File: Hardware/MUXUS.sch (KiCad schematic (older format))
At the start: 120 parts, among them J1 USB_C_Receptacle_USB2.0, J2 USB_B, J3 USB_A, J4 USB_B, J5 USB_A, J6 STDC14, J7 USB_B, J8 USB_A, SW1 USER, SW2 RESET, U1 USBLC6-4SC6, U10 AP2151W, U11 AOZ1212AI, U12 USBLC6-2SC6, U13 USBLC6-2SC6, U14 AP2151W, U2 USB2504A-JT, U3 USBLC6-2SC6, U4 USBLC6-2SC6, U5 AP2151W, U6 TS3USBCA420RSVR, U7 STM32G431K8T6, U8 USBLC6-2SC6, U9 USBLC6-2SC6, Y1 ATS240C

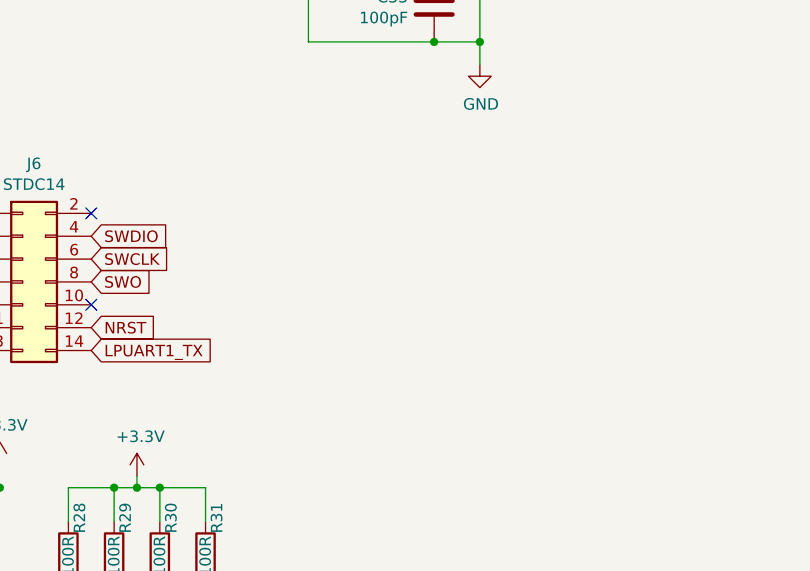
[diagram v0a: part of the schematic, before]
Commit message: DEBUG connectors and VIAS
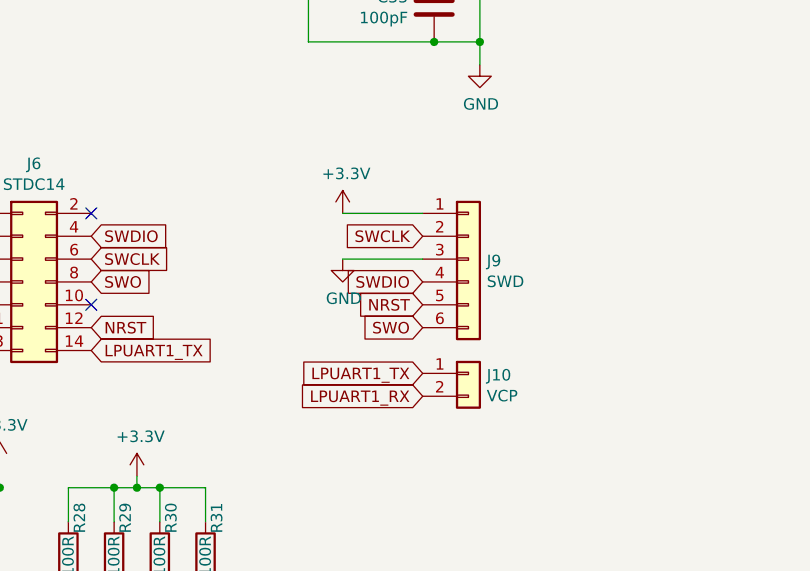
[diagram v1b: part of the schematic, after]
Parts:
- added J10: VCP, Connector_PinHeader_2.54mm:PinHeader_1x02_P2.54mm_Vertical, symbol Connector_Generic:Conn_01x02
- added J9: SWD, Connector_PinHeader_2.54mm:PinHeader_1x06_P2.54mm_Vertical, symbol Connector_Generic:Conn_01x06
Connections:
- net +3V3: now also J9.1 (Pin_1)
- net GND: now also J9.3 (Pin_3)
- net LPUART1_RX: now also J10.2 (Pin_2)
- net LPUART1_TX: now also J10.1 (Pin_1)
- net NRST: now also J9.5 (Pin_5)
- net SWCLK: now also J9.2 (Pin_2)
- net SWDIO: now also J9.4 (Pin_4)
- net SWO: now also J9.6 (Pin_6)
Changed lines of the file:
@@
 	2400 4350 2600 4350
 Connection ~ 2400 4650
+$Comp
+L Connector_Generic:Conn_01x06 J9
+U 1 1 615B40A3
+P 12450 8450
+F 0 "J9" H 12530 8442 50  0000 L CNN
+F 1 "SWD" H 12530 8351 50  0000 L CNN
+F 2 "Connector_PinHeader_2.54mm:PinHeader_1x06_P2.54mm_Vertical" H 12450 8450 50  0001 C CNN
+F 3 "~" H 12450 8450 50  0001 C CNN
+	1    12450 8450
+	1    0    0    -1
+$EndComp
+$Comp
+L Connector_Generic:Conn_01x02 J10
+U 1 1 615B75B8
+P 12450 8950
+F 0 "J10" H 12530 8942 50  0000 L CNN
+F 1 "VCP" H 12530 8851 50  0000 L CNN
+F 2 "Connector_PinHeader_2.54mm:PinHeader_1x02_P2.54mm_Vertical" H 12450 8950 50  0001 C CNN
+F 3 "~" H 12450 8950 50  0001 C CNN
+	1    12450 8950
+	1    0    0    -1
+$EndComp
+$Comp
+L power:+3.3V #PWR063
+U 1 1 615B80D0
+P 11900 8250
+F 0 "#PWR063" H 11900 8100 50  0001 C CNN
+F 1 "+3.3V" H 11915 8423 50  0000 C CNN
+F 2 "" H 11900 8250 50  0001 C CNN
+F 3 "" H 11900 8250 50  0001 C CNN
+	1    11900 8250
+	1    0    0    -1
+$EndComp
+Wire Wire Line
+	11900 8250 12250 8250
+Text GLabel 12250 8350 0    50   Input ~ 0
+SWCLK
+$Comp
+L power:GND #PWR064
+U 1 1 615DED53
+P 11900 8450
+F 0 "#PWR064" H 11900 8200 50  0001 C CNN
+F 1 "GND" H 11905 8277 50  0000 C CNN
+F 2 "" H 11900 8450 50  0001 C CNN
+F 3 "" H 11900 8450 50  0001 C CNN
+	1    11900 8450
+	1    0    0    -1
+$EndComp
+Wire Wire Line
+	11900 8450 12250 8450
+Text GLabel 12250 8550 0    50   Input ~ 0
+SWDIO
+Text GLabel 12250 8650 0    50   Input ~ 0
+NRST
+Text GLabel 12250 8750 0    50   Input ~ 0
+SWO
+Text GLabel 12250 8950 0    50   Input ~ 0
+LPUART1_TX
+Text GLabel 12250 9050 0    50   Input ~ 0
+LPUART1_RX
 $EndSCHEMATC
